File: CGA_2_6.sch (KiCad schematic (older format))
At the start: 4 parts, among them U34 74LS273, U35 74LS273, U36 74LS244, U37 74LS374

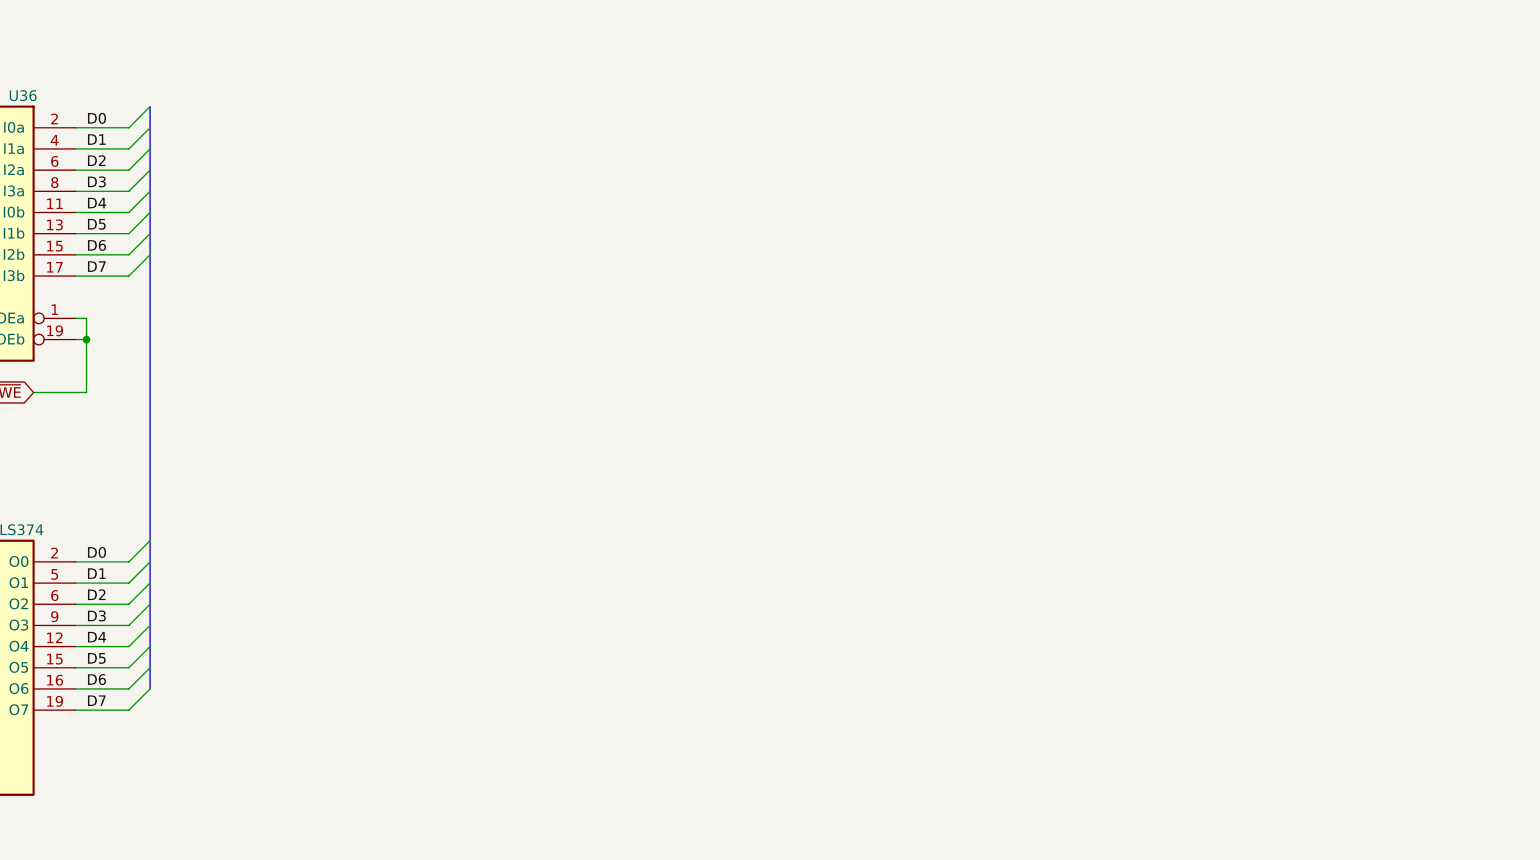
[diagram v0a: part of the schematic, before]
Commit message: More sheet 2
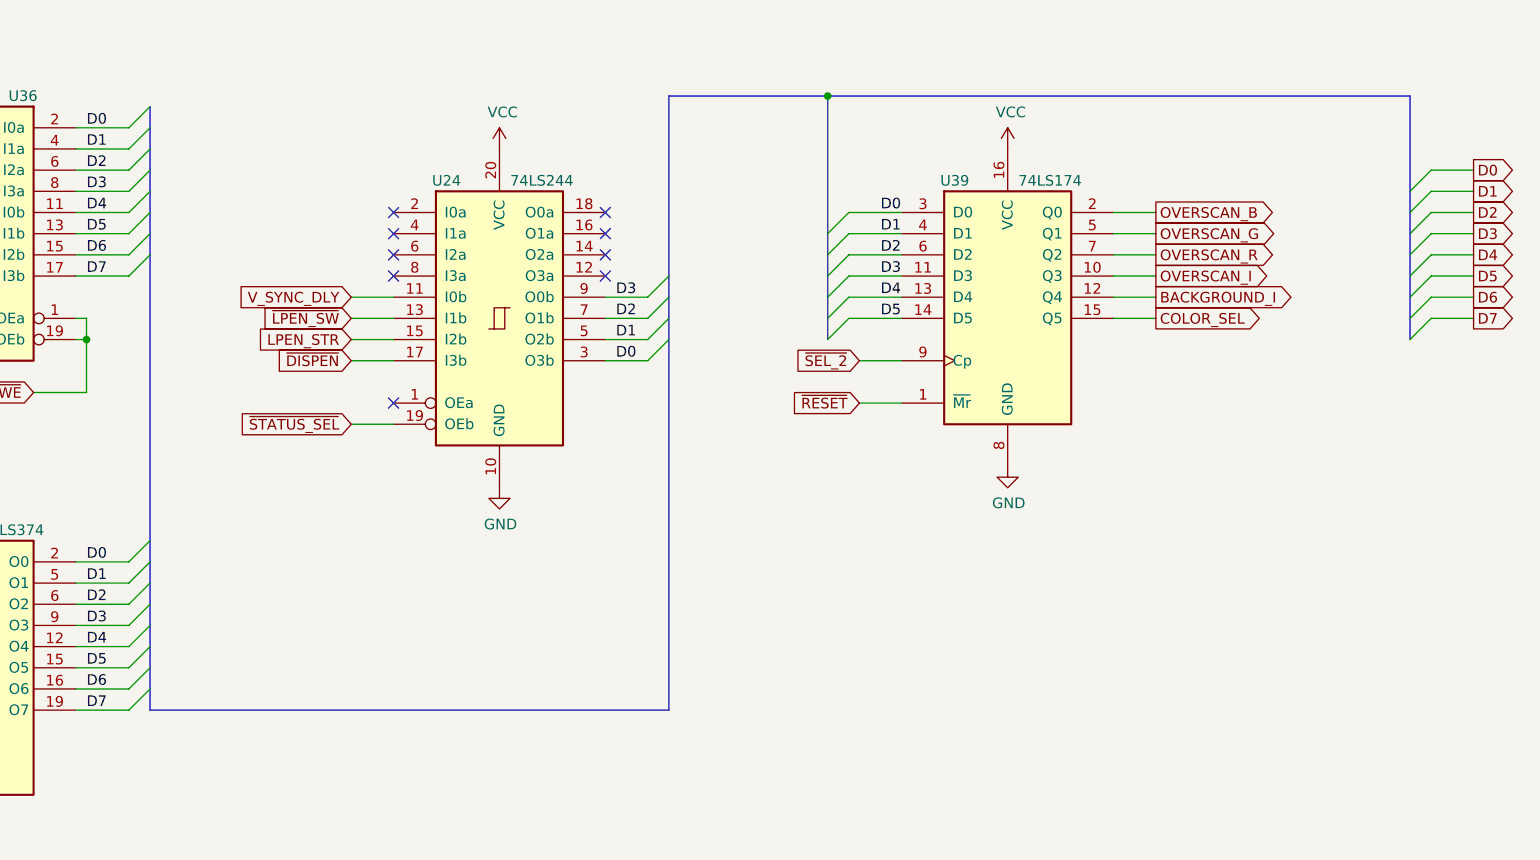
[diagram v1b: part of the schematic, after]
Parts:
- added U24: 74LS244, Package_DIP:DIP-20_W7.62mm_LongPads, symbol 74xx:74LS244
- added U39: 74LS174, Package_DIP:DIP-16_W7.62mm_LongPads, symbol 74xx:74LS174
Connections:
- net D0: now also U24.3 (O3b), U39.3 (D0)
- net D1: now also U24.5 (O2b), U39.4 (D1)
- net D2: now also U24.7 (O1b), U39.6 (D2)
- net D3: now also U24.9 (O0b), U39.11 (D3)
- net D4: now also U39.13 (D4)
- net D5: now also U39.14 (D5)
- net GND: now also U24.10 (GND), U39.8 (GND)
- net VCC: now also U24.20 (VCC), U39.16 (VCC)
- new net BACKGROUND_I: U39.12 (Q4)
- new net COLOR_SEL: U39.15 (Q5)
- new net LPEN_STR: U24.15 (I2b)
- new net OVERSCAN_B: U39.2 (Q0)
- new net OVERSCAN_G: U39.5 (Q1)
- new net OVERSCAN_I: U39.10 (Q3)
- new net OVERSCAN_R: U39.7 (Q2)
- new net V_SYNC_DLY: U24.11 (I0b)
- new net ~DISPEN: U24.17 (I3b)
- new net ~LPEN_SW: U24.13 (I1b)
- new net ~RESET: U39.1 (~Mr)
- new net ~SEL_2: U39.9 (Cp)
- new net ~STATUS_SEL: U24.19 (OEb)
- no-connect marks 0 -> 9

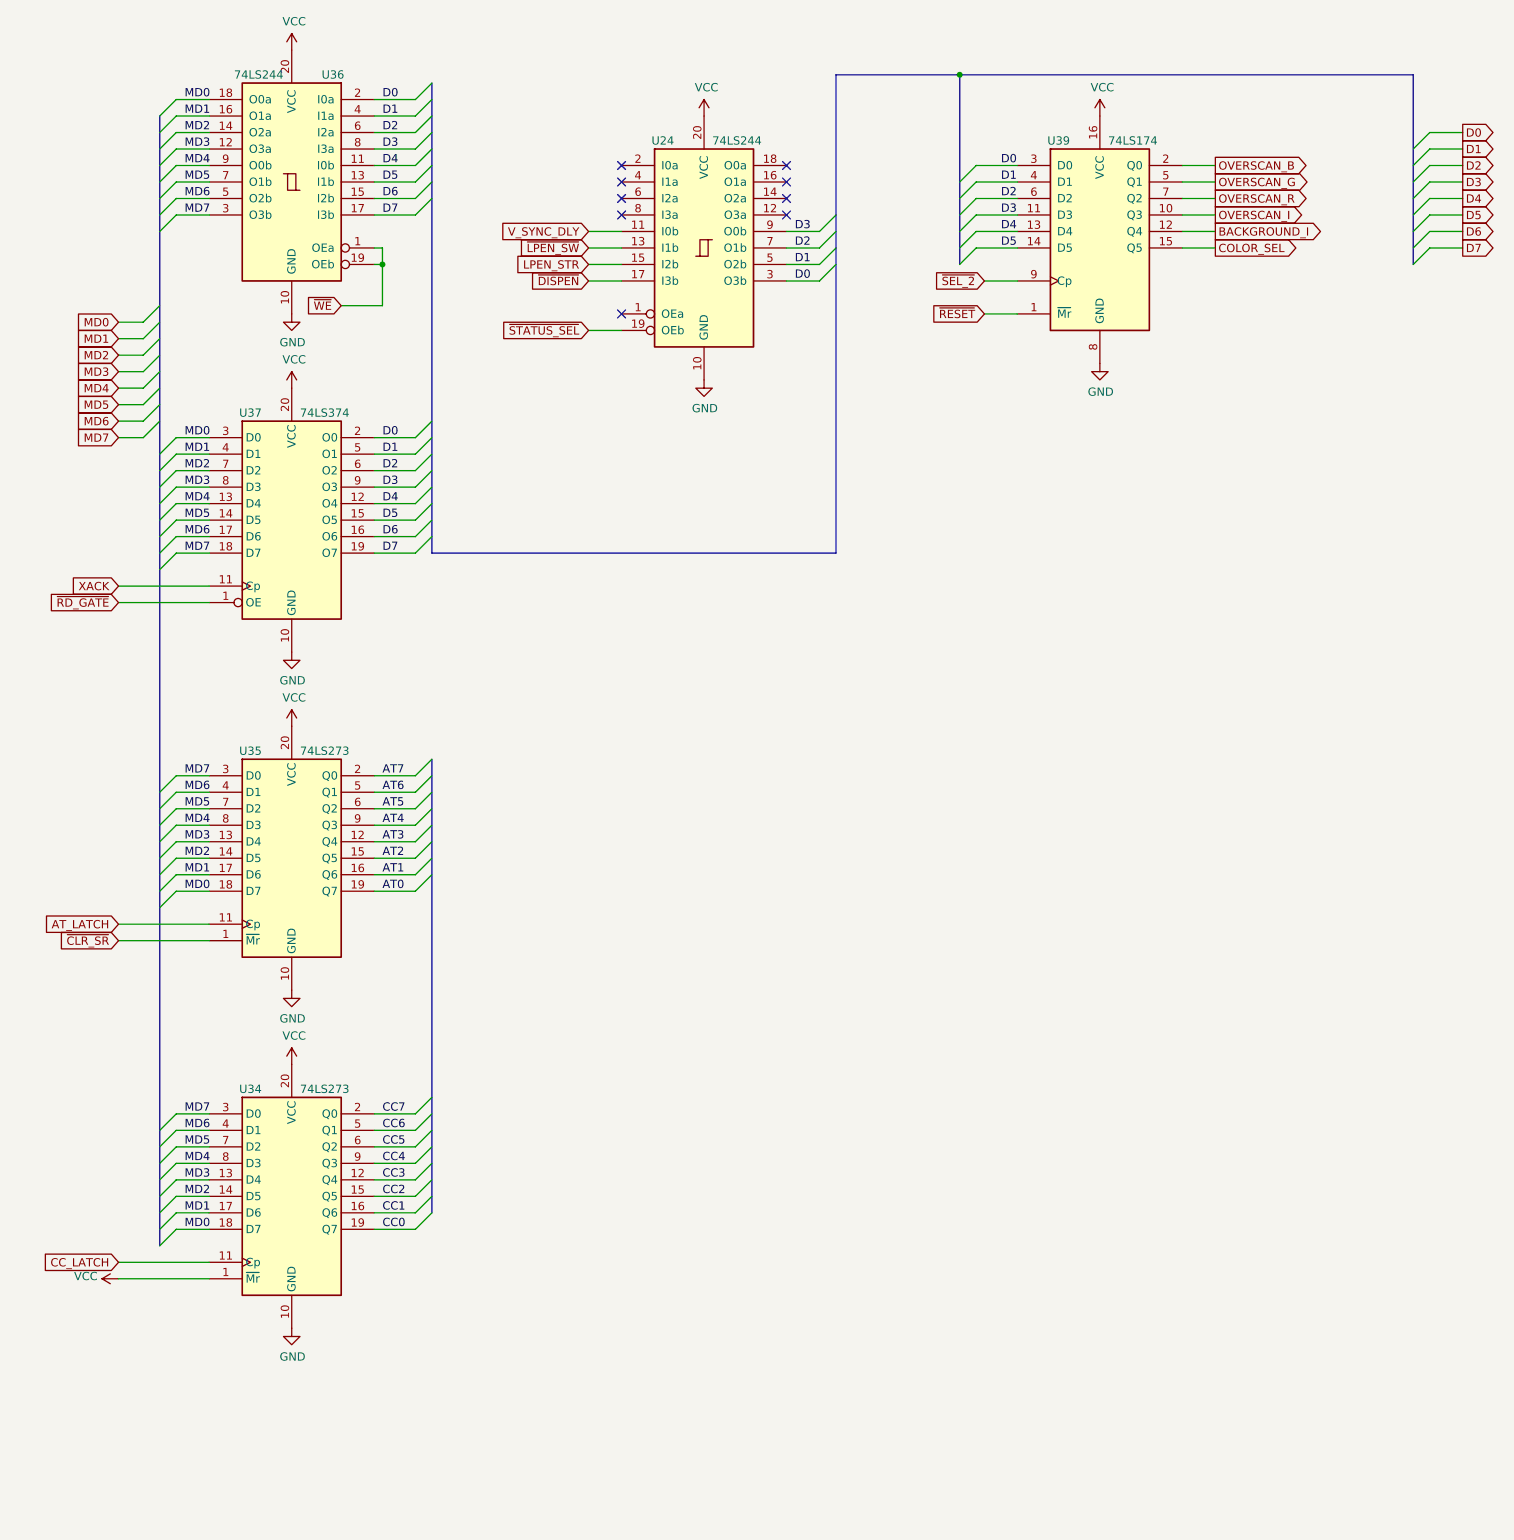
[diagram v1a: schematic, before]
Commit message: More sheet 2
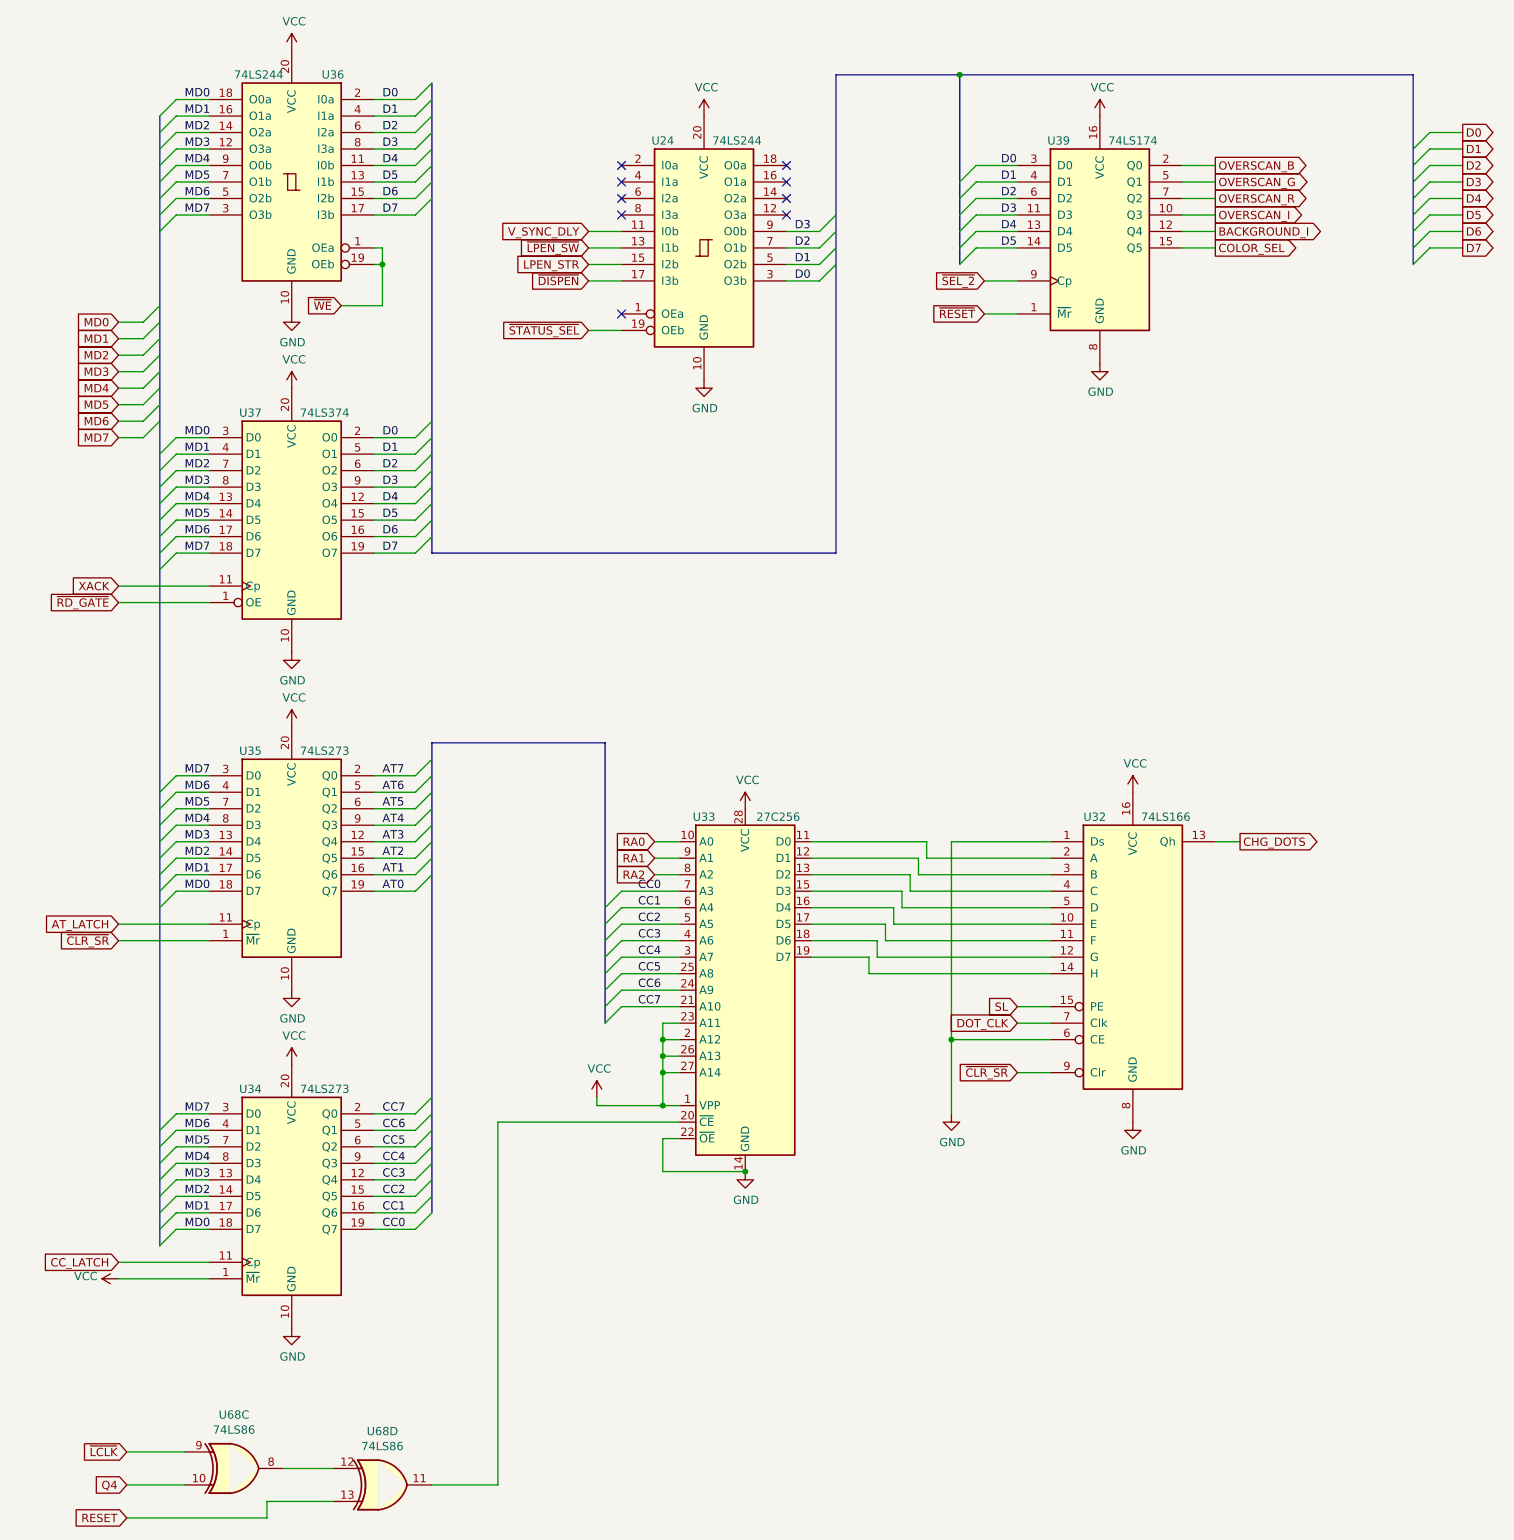
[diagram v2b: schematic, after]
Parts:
- added U32: 74LS166, Package_DIP:DIP-16_W7.62mm_LongPads, symbol 74xx:74LS166
- added U33: 27C256, Package_DIP:DIP-28_W15.24mm_LongPads, symbol Memory_EPROM:27C256
- added U68: 74LS86, Package_DIP:DIP-14_W7.62mm_LongPads, symbol 74xx:74LS86
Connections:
- net CC0: now also U33.7 (A3)
- net CC1: now also U33.6 (A4)
- net CC2: now also U33.5 (A5)
- net CC3: now also U33.4 (A6)
- net CC4: now also U33.3 (A7)
- net CC5: now also U33.25 (A8)
- net CC6: now also U33.24 (A9)
- net CC7: now also U33.21 (A10)
- net GND: now also U32.1 (Ds), U32.6 (CE), U32.8 (GND), U33.14 (GND), U33.22 (~OE)
- net VCC: now also U32.16 (VCC), U33.1 (VPP), U33.2 (A12), U33.23 (A11), U33.26 (A13), U33.27 (A14), U33.28 (VCC)
- net ~CLR_SR: now also U32.9 (Clr)
- new net: U32.2 (A), U33.11 (D0)
- new net: U32.3 (B), U33.12 (D1)
- new net: U32.4 (C), U33.13 (D2)
- new net: U32.5 (D), U33.15 (D3)
- new net: U32.10 (E), U33.16 (D4)
- new net: U32.11 (F), U33.17 (D5)
- new net: U32.12 (G), U33.18 (D6)
- new net: U32.14 (H), U33.19 (D7)
- new net: U33.20 (~CE), U68.11
- new net: U68.12, U68.8
- new net CHG_DOTS: U32.13 (Qh)
- new net DOT_CLK: U32.7 (Clk)
- new net Q4: U68.10
- new net RA0: U33.10 (A0)
- new net RA1: U33.9 (A1)
- new net RA2: U33.8 (A2)
- new net RESET: U68.13
- new net SL: U32.15 (PE)
- new net ~LCLK: U68.9
